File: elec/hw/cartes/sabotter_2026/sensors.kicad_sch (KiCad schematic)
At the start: 32 parts, among them J17 22272061, J5 22272041, U4 ADXRS453BRGZ, U5 SCH16T-K01-10

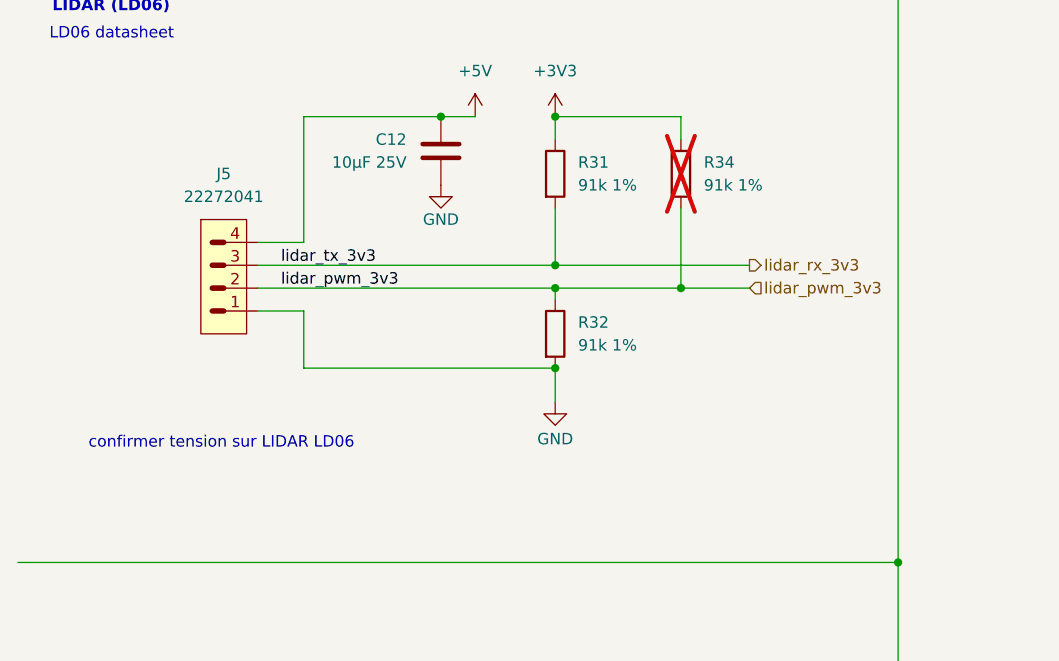
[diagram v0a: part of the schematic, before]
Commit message: sabotter wip
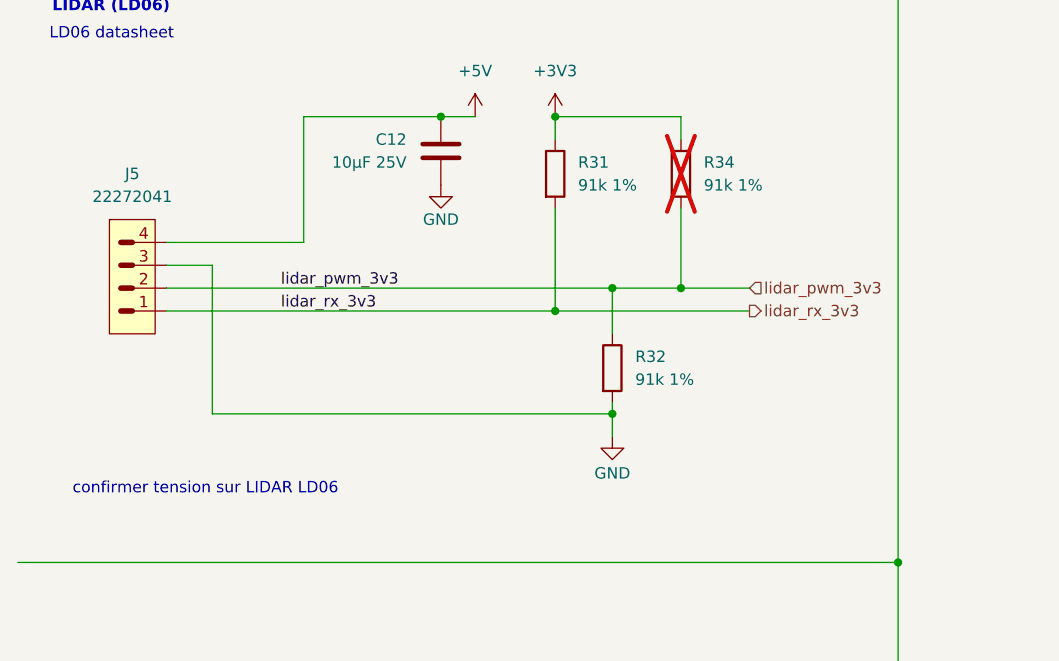
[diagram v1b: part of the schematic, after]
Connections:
- net GND: now also J5.3; no longer J5.1
- net lidar_rx_3v3: now also J5.1; no longer J5.3, R28.2, R30.2
- new net lidar_tx_3v3: R28.2, R30.2
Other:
- moved on the sheet: J5, R32
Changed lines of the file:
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@@
 	)
 	(junction
+		(at 80.01 118.11)
+		(diameter 0)
+		(color 0 0 0 0)
+	)
+	(junction
 		(at 204.47 73.66)
 		(diameter 0)
@@
 	)
 	(junction
-		(at 73.66 115.57)
-		(diameter 0)
-		(color 0 0 0 0)
-	)
-	(junction
 		(at 168.91 19.05)
 		(diameter 0)
@@
 	)
 	(junction
+		(at 73.66 120.65)
+		(diameter 0)
+		(color 0 0 0 0)
+	)
+	(junction
 		(at 179.07 73.66)
 		(diameter 0)
@@
 	)
 	(junction
-		(at 73.66 118.11)
-		(diameter 0)
-		(color 0 0 0 0)
-	)
-	(junction
 		(at 72.39 74.93)
 		(diameter 0)
@@
 	)
 	(junction
-		(at 73.66 127)
+		(at 196.85 73.66)
 		(diameter 0)
 		(color 0 0 0 0)
 	)
 	(junction
-		(at 196.85 73.66)
+		(at 60.96 99.06)
 		(diameter 0)
 		(color 0 0 0 0)
 	)
 	(junction
-		(at 60.96 99.06)
+		(at 80.01 132.08)
 		(diameter 0)
 		(color 0 0 0 0)
@@
 	(wire
 		(pts
-			(xy 227.33 25.4) (xy 245.11 25.4)
+			(xy 30.48 120.65) (xy 73.66 120.65)
 		)
 		(stroke
@@
 	(wire
 		(pts
-			(xy 204.47 73.66) (xy 207.01 73.66)
+			(xy 227.33 25.4) (xy 245.11 25.4)
 		)
 		(stroke
@@
 	(wire
 		(pts
-			(xy 203.2 24.13) (xy 203.2 17.78)
+			(xy 204.47 73.66) (xy 207.01 73.66)
 		)
 		(stroke
@@
 	(wire
 		(pts
-			(xy 203.2 17.78) (xy 205.74 17.78)
+			(xy 203.2 24.13) (xy 203.2 17.78)
 		)
 		(stroke
@@
 	(wire
 		(pts
-			(xy 168.91 69.85) (xy 168.91 73.66)
+			(xy 203.2 17.78) (xy 205.74 17.78)
 		)
 		(stroke
@@
 	(wire
 		(pts
-			(xy 73.66 109.22) (xy 73.66 115.57)
+			(xy 168.91 69.85) (xy 168.91 73.66)
 		)
 		(stroke
@@
 	(wire
 		(pts
-			(xy 40.64 115.57) (xy 73.66 115.57)
-		)
-		(stroke
-			(width 0)
-			(type default)
-		)
-	)
-	(wire
-		(pts
 			(xy 68.58 177.8) (xy 86.36 177.8)
 		)
@@
 	(wire
 		(pts
+			(xy 80.01 130.81) (xy 80.01 132.08)
+		)
+		(stroke
+			(width 0)
+			(type default)
+		)
+	)
+	(wire
+		(pts
 			(xy 85.09 74.93) (xy 87.63 74.93)
 		)
@@
 	(wire
 		(pts
-			(xy 13.97 85.09) (xy 111.76 85.09)
+			(xy 30.48 118.11) (xy 80.01 118.11)
 		)
 		(stroke
 			(width 0)
-			(type dash)
+			(type default)
 		)
 	)
 	(wire
 		(pts
-			(xy 45.72 127) (xy 45.72 120.65)
+			(xy 13.97 85.09) (xy 111.76 85.09)
 		)
 		(stroke
 			(width 0)
-			(type default)
+			(type dash)
 		)
 	)
@@
 	(wire
 		(pts
-			(xy 40.64 118.11) (xy 73.66 118.11)
-		)
-		(stroke
-			(width 0)
-			(type default)
-		)
-	)
-	(wire
-		(pts
 			(xy 217.17 36.83) (xy 218.44 36.83)
 		)
@@
 	(wire
 		(pts
-			(xy 95.25 115.57) (xy 73.66 115.57)
+			(xy 95.25 120.65) (xy 73.66 120.65)
 		)
 		(stroke
@@
 	(wire
 		(pts
+			(xy 35.56 132.08) (xy 80.01 132.08)
+		)
+		(stroke
+			(width 0)
+			(type default)
+		)
+	)
+	(wire
+		(pts
 			(xy 207.01 71.12) (xy 207.01 73.66)
 		)
@@
 	(wire
 		(pts
-			(xy 73.66 130.81) (xy 73.66 127)
+			(xy 80.01 134.62) (xy 80.01 132.08)
 		)
 		(stroke
@@
 	(wire
 		(pts
-			(xy 218.44 54.61) (xy 224.79 54.61)
+			(xy 30.48 113.03) (xy 45.72 113.03)
 		)
 		(stroke
@@
 	(wire
 		(pts
-			(xy 82.55 74.93) (xy 85.09 74.93)
+			(xy 218.44 54.61) (xy 224.79 54.61)
 		)
 		(stroke
@@
 	(wire
 		(pts
-			(xy 77.47 74.93) (xy 82.55 74.93)
+			(xy 82.55 74.93) (xy 85.09 74.93)
 		)
 		(stroke
@@
 	(wire
 		(pts
-			(xy 45.72 120.65) (xy 40.64 120.65)
+			(xy 77.47 74.93) (xy 82.55 74.93)
 		)
 		(stroke
@@
 	(wire
 		(pts
-			(xy 73.66 118.11) (xy 73.66 119.38)
+			(xy 80.01 118.11) (xy 80.01 123.19)
 		)
 		(stroke
@@
 	(wire
 		(pts
-			(xy 73.66 127) (xy 45.72 127)
+			(xy 30.48 115.57) (xy 35.56 115.57)
 		)
 		(stroke
@@
 	(wire
 		(pts
+			(xy 35.56 115.57) (xy 35.56 132.08)
+		)
+		(stroke
+			(width 0)
+			(type default)
+		)
+	)
+	(wire
+		(pts
 			(xy 156.21 46.99) (xy 184.15 46.99)
 		)
@@
 	(wire
 		(pts
-			(xy 87.63 118.11) (xy 73.66 118.11)
+			(xy 87.63 118.11) (xy 80.01 118.11)
 		)
 		(stroke
@@
 	(wire
 		(pts
-			(xy 45.72 113.03) (xy 40.64 113.03)
+			(xy 73.66 109.22) (xy 73.66 120.65)
 		)
 		(stroke
@@
 	(text "confirmer tension sur LIDAR LD06"
 		(exclude_from_sim no)
-		(at 36.576 135.382 0)
+		(at 34.798 140.462 0)
 		(effects
 			(font
@@
 		)
 	)
-	(label "lidar_tx_3v3"
-		(at 43.18 115.57 0)
+	(label "lidar_rx_3v3"
+		(at 43.18 120.65 0)
 		(effects
 			(font
@@
 	(hierarchical_label "lidar_rx_3v3"
 		(shape output)
-		(at 95.25 115.57 0)
+		(at 95.25 120.65 0)
 		(effects
 			(font
@@
 	(symbol
 		(lib_id "power:GND")
-		(at 73.66 130.81 0)
+		(at 80.01 134.62 0)
 		(mirror y)
 		(unit 1)
@@
 		(dnp no)
 		(property "Reference" "#PWR34"
-			(at 73.66 137.16 0)
+			(at 80.01 140.97 0)
 			(effects
 				(font
@@
 		)
 		(property "Value" "GND"
-			(at 73.66 134.874 0)
+			(at 80.01 138.684 0)
 			(effects
 				(font
@@
 		)
 		(property "Footprint" ""
-			(at 73.66 130.81 0)
+			(at 80.01 134.62 0)
 			(effects
 				(font
@@
 		)
 		(property "Datasheet" ""
-			(at 73.66 130.81 0)
+			(at 80.01 134.62 0)
 			(effects
 				(font
@@
 		)
 		(property "Description" "Power symbol creates a global label with name \"GND\" , ground"
-			(at 73.66 130.81 0)
+			(at 80.01 134.62 0)
 			(effects
 				(font
@@
 	(symbol
 		(lib_id "cocotter_connectors:22272041")
-		(at 40.64 118.11 0)
+		(at 30.48 118.11 0)
 		(unit 1)
 		(exclude_from_sim no)
@@
 		(fields_autoplaced yes)
 		(property "Reference" "J5"
-			(at 36.83 105.41 0)
+			(at 26.67 105.41 0)
 			(effects
 				(font
@@
 		)
 		(property "Value" "22272041"
-			(at 36.83 107.95 0)
+			(at 26.67 107.95 0)
 			(effects
 				(font
@@
 		)
 		(property "Footprint" "cocotter_connectors:22272041"
-			(at 37.338 130.048 0)
+			(at 27.178 130.048 0)
 			(effects
 				(font
@@
 		)
 		(property "Datasheet" "https://www.molex.com/en-us/products/part-detail/22272041"
-			(at 40.64 127 0)
+			(at 30.48 127 0)
 			(effects
 				(font
@@
 		)
 		(property "Description" "mini kk 4 voies vertical"
-			(at 40.64 127 0)
+			(at 30.48 127 0)
 			(effects
 				(font
@@
 	(symbol
 		(lib_id "cocotter_resistors:R_91k_0603_1%")
-		(at 73.66 123.19 0)
+		(at 80.01 127 0)
 		(unit 1)
 		(exclude_from_sim no)
@@
 		(fields_autoplaced yes)
 		(property "Reference" "R32"
-			(at 76.2 121.9199 0)
+			(at 82.55 125.7299 0)
 			(effects
 				(font
@@
 		)
 		(property "Value" "91k 1%"
-			(at 76.2 124.4599 0)
+			(at 82.55 128.2699 0)
 			(effects
 				(font
@@
 		)
 		(property "Footprint" "cocotter_resistor:r0603_reflow"
-			(at 71.882 123.19 90)
+			(at 78.232 127 90)
 			(effects
 				(font
@@
 		)
 		(property "Datasheet" "~"
-			(at 73.66 123.19 0)
+			(at 80.01 127 0)
 			(effects
 				(font
@@
 		)
 		(property "Description" "Resistor"
-			(at 73.66 123.19 0)
+			(at 80.01 127 0)
 			(effects
 				(font
@@
 		)
 		(property "Specification" "91k 0603 1% 100mW"
-			(at 73.66 123.19 0)
+			(at 80.01 127 0)
 			(effects
 				(font
@@
 		)
 		(property "mouser" ""
-			(at 73.66 123.19 0)
+			(at 80.01 127 0)
 			(effects
 				(font
@@
 		)
 		(property "JLCPCB Part #" "C23265"
-			(at 73.66 123.19 0)
+			(at 80.01 127 0)
 			(effects
 				(font
